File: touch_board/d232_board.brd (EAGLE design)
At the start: 116.5 x 80 mm, 30 parts, among them IC1 uln2803, IC2 uln2803, IC3 7805TV, IC4 7805TV, IC5 7805TV, X1 057-050-1

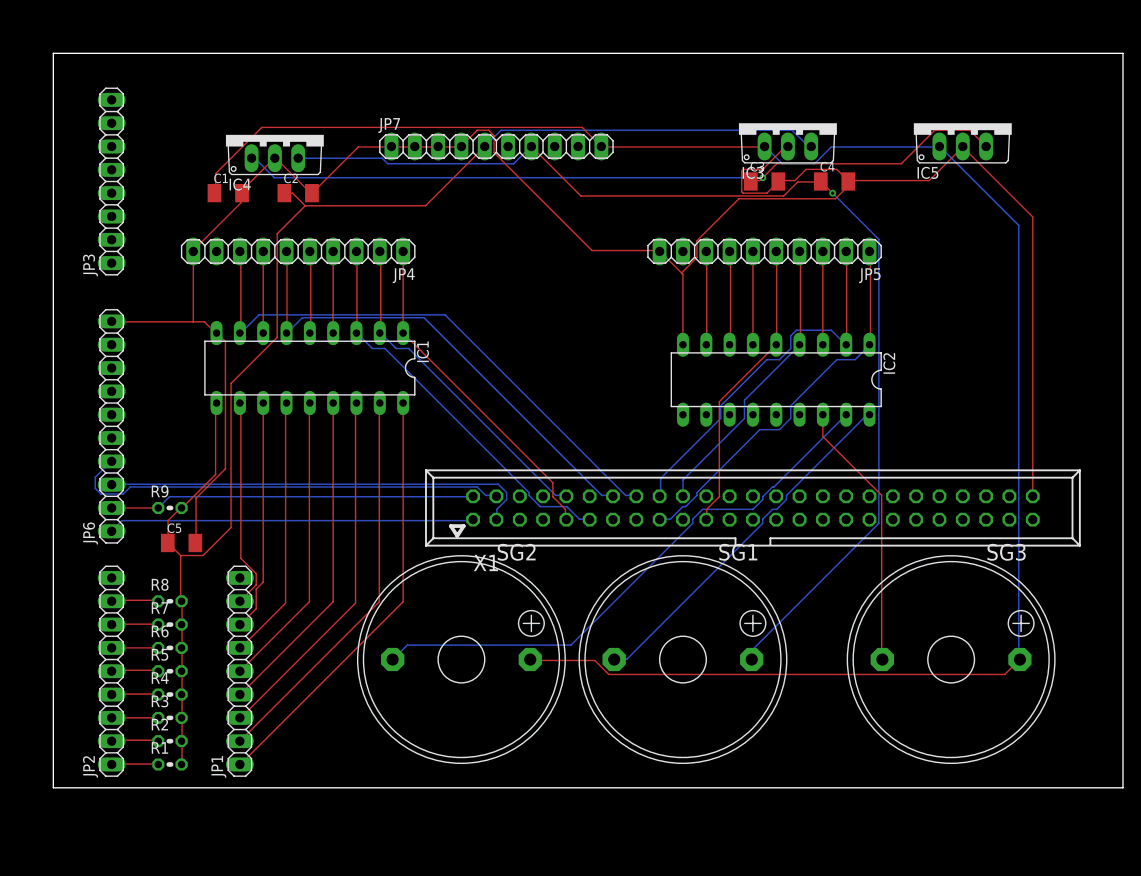
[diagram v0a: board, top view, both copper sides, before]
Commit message: up
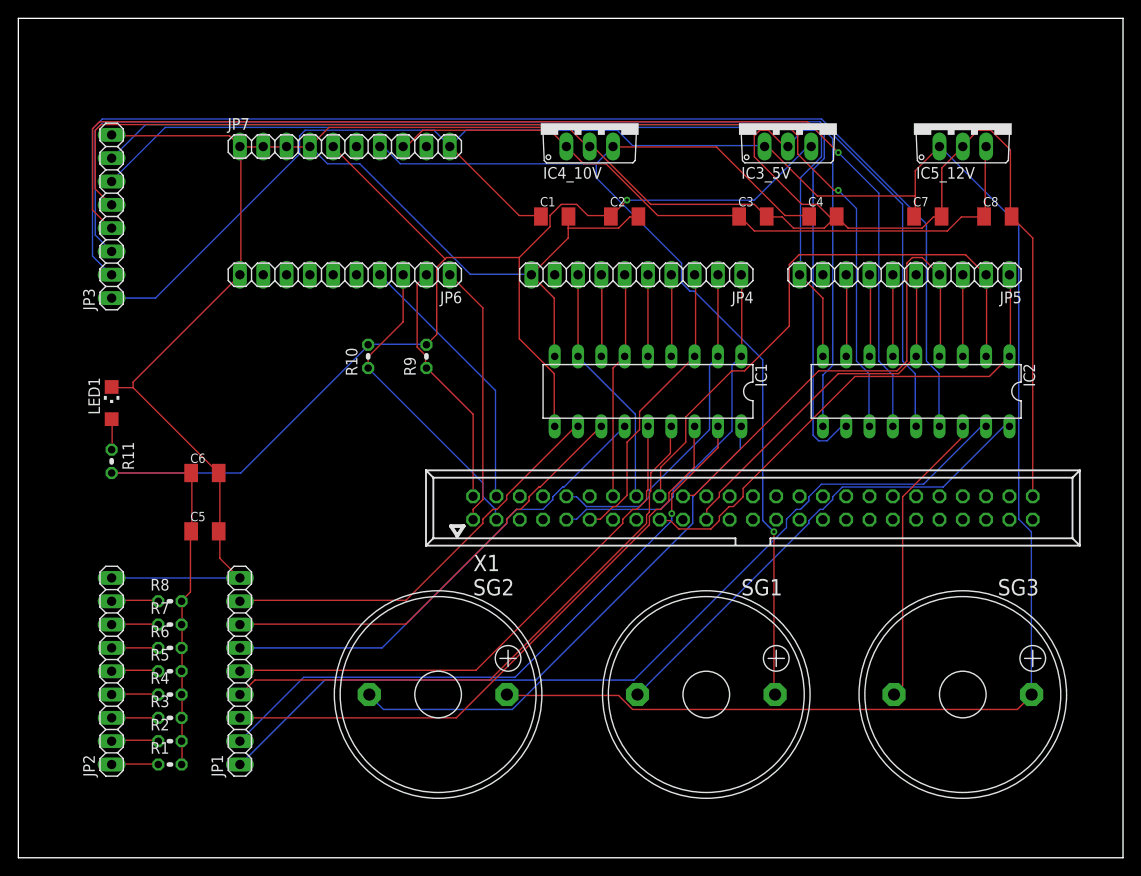
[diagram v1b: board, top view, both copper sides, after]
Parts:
- removed IC4: 7805TV, linear:TO220V
- added C6, C7: 0.47, rcl:C1206K
- added C8: 22uf, rcl:C1206K
- added IC4_10V: 7805TV, linear:TO220V
- added LED1: PWR, led:CHIPLED_1206
- added R10: 91, rcl:0204V
- added R11: 1k, rcl:0204V
- JP1: value (none) -> LEDC
- JP2: value (none) -> LEDP
- JP3: value (none) -> PORTIO
- JP4: value (none) -> PORT2
- JP5: value (none) -> PORT3
- JP6: value (none) -> PORT1
- JP7: value (none) -> DC POWER
- moved IC1 36.9 mm to (64.8, 43.2)
- moved JP4 36.9 mm to (63.5, 55.9)
- moved C1 35.7 mm to (54.6, 62.2)
- moved C2 35.7 mm to (62.2, 62.2)
- moved R9 32.5 mm to (40.6, 47.0), turned to 90 degrees
- moved JP6 30.3 mm to (31.8, 55.9), turned to 180 degrees
- moved JP7 16.5 mm to (31.8, 69.8)
- moved JP5 15.5 mm to (92.7, 55.9)
- moved IC2 15.3 mm to (94.0, 43.2)
- moved SG1 4.58 mm to (71.1, 10.2)
- moved SG2 4.58 mm to (41.9, 10.2)
- moved C4 4.02 mm to (83.8, 62.2)
- moved C3 4.02 mm to (76.2, 62.2)
- moved SG3 4.02 mm to (99.1, 10.2)
- moved JP3 3.81 mm to (6.35, 62.2)
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- renumbered IC3 to IC3_5V, IC5 to IC5_12V
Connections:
- new net N$40: IC2.15, JP3.2
- new net N$41: IC2.14, JP3.3
- new net N$42: IC2.13, JP3.4
- new net N$43: IC2.12, JP3.5
- new net N$44: IC2.11, JP3.6
- new net N$45: IC2.10, JP3.7
- new net N$46: LED1.A, R11.1
- net +10V: now also IC4_10V.3; no longer IC4.3
- net +12V: now also C8.1, IC4_10V.1, JP7.8; no longer IC4.1
- net +24V: now also C7.1, JP3.1
- net +5V: now also C6.1, R10.2, R11.2
- net GND: now also C6.2, C7.2, C8.2, IC4_10V.2, JP1.9, JP2.9, JP3.8, LED1.C; no longer IC4.2
- net N$30: now also R10.1
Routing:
- net N$40: track 0.00 -> 135.4 mm
- net N$41: track 0.00 -> 130.8 mm
- net N$42: track 0.00 -> 127.0 mm, vias 0 -> 1
- net N$43: track 0.00 -> 121.3 mm, vias 0 -> 1
- net N$44: track 0.00 -> 118.2 mm
- net N$45: track 0.00 -> 112.5 mm
- net GND: track 223.2 -> 331.3 mm
- net +24V: track 199.9 -> 245.0 mm
- net N$16: track 61.2 -> 26.8 mm
- net N$14: track 53.3 -> 24.7 mm
- net N$5: track 32.4 -> 60.3 mm
- net N$4: track 36.0 -> 63.7 mm
- net N$3: track 39.7 -> 66.3 mm
- net N$1: track 46.8 -> 73.0 mm
- net N$2: track 43.2 -> 69.3 mm, vias 0 -> 1
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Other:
- board size 116.5 x 80 mm -> 120.3 x 91.4 mm
